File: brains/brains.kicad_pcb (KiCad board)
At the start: 2 copper layers, 86.4 x 55.9 mm, 22 parts, among them U1 WiiChuckCon, U10 Servo, U11 Servo, U12 Servo, U13 XBEE, U2 Nokia_5510_LCD, U3 promicro, U4 JoyConnectISP, U5 JACK_2MM1, U6 TXB0108PWR, U7 HM-11_Bluetooth, U8 AP1117_V_REG, U9 Servo

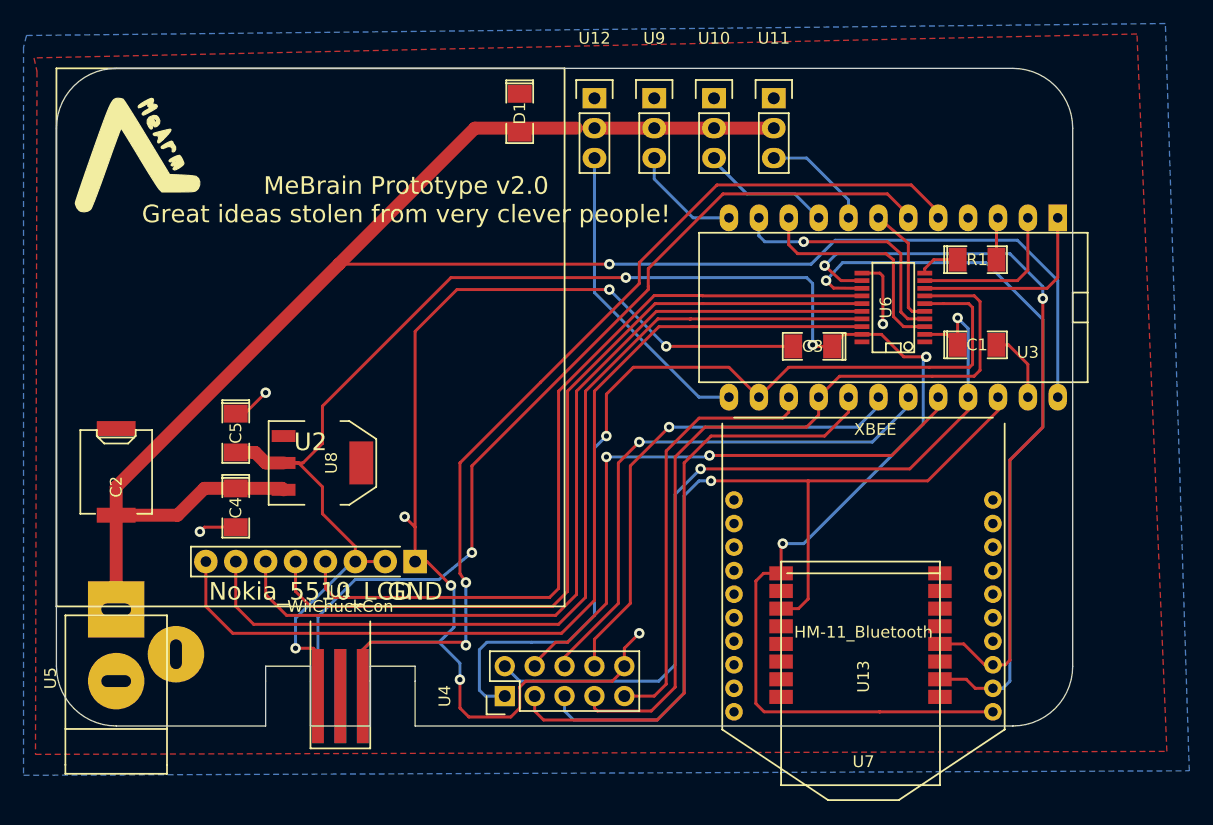
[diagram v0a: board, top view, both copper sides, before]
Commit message: V1.0 Update
Kickstarter Production version
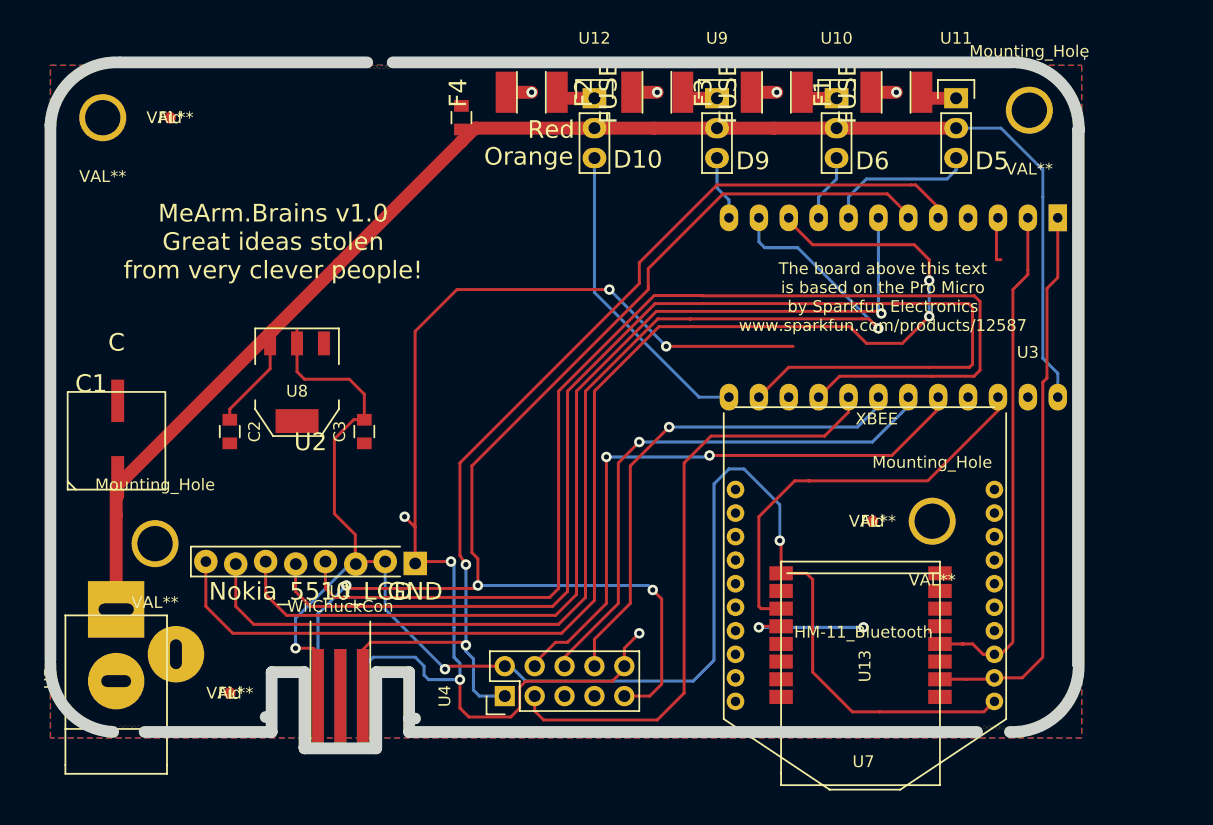
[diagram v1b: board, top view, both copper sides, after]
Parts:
- removed the ? at (98.8, 80.0)
- removed the ? at (148.8, 101.6)
- removed C5: C, SMD_Packages:SMD-1206_Pol
- removed D1: DIODE, SMD_Packages:SMD-1206_Pol
- removed R1: R, SMD_Packages:SMD-1206_Pol
- removed U6: TXB0108PWR, SMD_Packages:SSOP-20
- added ?: , Brains:TinyDrillHole, F.Cu at (98.9, 128.7)
- added ?: , TinyDrillHole, F.Cu at (170.8, 128.7)
- added ?: , TinyDrillHole, F.Cu at (118.6, 72.5)
- added ?: VAL**, Brains:Mounting_Hole, F.Cu at (95.9, 76.8)
- added ?: , Brains:TinyDrillHole, F.Cu at (119.0, 72.5)
- added ?: , Brains:TinyDrillHole, F.Cu at (119.4, 72.5)
- added ?: , Brains:TinyDrillHole, F.Cu at (119.8, 72.5)
- added ?: , Brains:TinyDrillHole, F.Cu at (120.1, 72.5)
- added ?: , Brains:TinyDrillHole, F.Cu at (98.6, 128.7)
- added ?: , Brains:TinyDrillHole, F.Cu at (98.2, 128.7)
- added ?: , Brains:TinyDrillHole, F.Cu at (97.8, 128.7)
- added ?: , TinyDrillHole, F.Cu at (97.4, 128.7)
- added ?: , Brains:TinyDrillHole, F.Cu at (172.3, 128.7)
- added ?: , Brains:TinyDrillHole, F.Cu at (172.0, 128.7)
- added ?: , Brains:TinyDrillHole, F.Cu at (171.6, 128.7)
- added ?: , Brains:TinyDrillHole, F.Cu at (171.2, 128.7)
- added F1: FUSE, Brains:Surface_Mount_1812_Polyfuse, F.Cu at (163.3, 74.7)
- added F2: FUSE, Brains:Surface_Mount_1812_Polyfuse, F.Cu at (143.0, 74.7)
- added F3: FUSE, Brains:Surface_Mount_1812_Polyfuse, F.Cu at (153.2, 74.7)
- added F4: FUSE, Brains:Surface_Mount_1812_Polyfuse, F.Cu at (132.3, 74.7)
- added Fid: VAL**, Fid, F.Cu at (101.6, 76.8)
- added Fid: VAL**, Brains:Fid, F.Cu at (106.7, 125.7)
- added Fid: VAL**, Brains:Fid, F.Cu at (161.3, 111.1)
- added Mounting_Hole: VAL**, Brains:Mounting_Hole, F.Cu at (174.6, 76.2)
- added Mounting_Hole: VAL**, Brains:Mounting_Hole, F.Cu at (100.3, 113.0)
- added Mounting_Hole: VAL**, Brains:Mounting_Hole, F.Cu at (166.4, 111.1)
- C1: footprint SMD_Packages:SMD-1206_Pol -> Brains:EEE1CA471UP_Capacitor
- C2: value C -> 10uF; footprint SMD_Packages:SMD-4032 -> Capacitors_SMD:C_0805
- C3: value C -> 22uF; footprint SMD_Packages:SMD-1206_Pol -> Capacitors_SMD:C_0805
- C4: footprint SMD_Packages:SMD-1206_Pol -> Capacitors_SMD:C_0805
- U1: footprint Brains:WiiChuck -> WiiChuck
- U10, U11, U12, U9: value Servo -> (none)
- moved C1 73.5 mm to (97.2, 104.1), turned to 180 degrees
- moved C3 38.8 mm to (118.1, 103.5), turned to 90 degrees
- moved C4 38.3 mm to (126.4, 76.8), turned to 90 degrees
- moved U11 15.5 mm to (168.4, 75.2)
- moved U10 10.4 mm to (158.2, 75.2)
- moved C2 10.2 mm to (106.7, 103.5), turned to 270 degrees
- moved U8 7.19 mm to (112.4, 99.3), turned to 180 degrees
- moved U9 5.33 mm to (148.1, 75.2)
- moved U13 0.90 mm to (160.7, 114.9)
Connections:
- C1 pad 1: +5V -> +6V
- C3 pad 1: +3V3 -> GND
- C3 pad 2: GND -> +3V3
- U10 pad 1: GND -> Net-(F2-Pad1)
- U11 pad 1: GND -> Net-(F3-Pad1)
- U12 pad 1: GND -> Net-(F4-Pad1)
- U13 pad 2: 3V_BT_TX -> BT_TX
- U13 pad 3: 3V_BT_RX -> BT_RX
- U2 pad 1: 3V_LCD_RST -> LCD_RST
- U2 pad 2: 3V_LCD_CE -> LCD_CE
- U2 pad 3: 3V_LCD_DC -> LCD_DC
- U2 pad 4: 3V_MOSI_D16 -> MOSI_D16
- U2 pad 5: 3V_SCLK_D15 -> SCLK_D15
- U3 pad 21: +5V -> Net-(U3-Pad21)
- U4 pad 1: MOSI_D16 -> I2C_SDA
- U4 pad 2: +5V -> +3V3
- U4 pad 5: RST -> GND
- U4 pad 7: SCLK_D15 -> GND
- U4 pad 9: MISO_D14 -> I2C_SCLK
- U7 pad 2: 3V_BT_TX -> BT_TX
- U7 pad 4: 3V_BT_RX -> BT_RX
- U9 pad 1: GND -> Net-(F1-Pad1)
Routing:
- net LCD_RST: track 19.5 -> 107.4 mm, vias 0 -> 2
- net 3V_LCD_RST: track 81.7 -> 0.00 mm
- net 3V_LCD_CE: track 78.7 -> 0.00 mm
- net 3V_LCD_DC: track 75.0 -> 0.00 mm
- net LCD_DC: track 10.3 -> 85.0 mm, vias 0 -> 1
- net LCD_CE: track 21.4 -> 95.7 mm
- net 3V_MOSI_D16: track 71.8 -> 0.00 mm
- net +5V: track 71.6 -> 0.00 mm, vias 2 -> 0
- net 3V_SCLK_D15: track 68.7 -> 0.00 mm
- net 3V_BT_RX: track 63.5 -> 0.00 mm, vias 2 -> 0
- net 3V_BT_TX: track 62.8 -> 0.00 mm, vias 1 -> 0
- net RST: track 74.0 -> 35.9 mm, vias 1 -> 0
- net MISO_D14: track 36.8 -> 0.00 mm
- net BT_TX: track 16.8 -> 47.3 mm
- net SCLK_D15: track 69.0 -> 99.4 mm
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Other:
- board size 86.4 x 55.9 mm -> 87.9 x 58.8 mm
- copper layers 2 -> 4
- board text added: "D10"
- board text added: "D5"
- board text added: "D6"
- board text added: "D9"
- board text added: "MeArm Limited 2015 CC-BY-SA 3.0"
- board text added: "MeArm.Brains v1.0 Great ideas stolen from very clever people!"
- board text added: "Orange"
- board text added: "Red"
- board text added: "The board above this text is based on the Pro Micro by Sparkfun Electronics www.sparkfun.com/products/12587"
- board text added: "With thanks to: Jack Howard, Ben Pirt, Arduino, Sparkfun, Adafruit, KiCad and everyone who shares their ideas and enthusiam."
- board text removed: "MeBrain Prototype v2.0 Great ideas stolen from very clever people!"
